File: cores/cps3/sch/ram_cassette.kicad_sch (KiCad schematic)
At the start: 13 parts

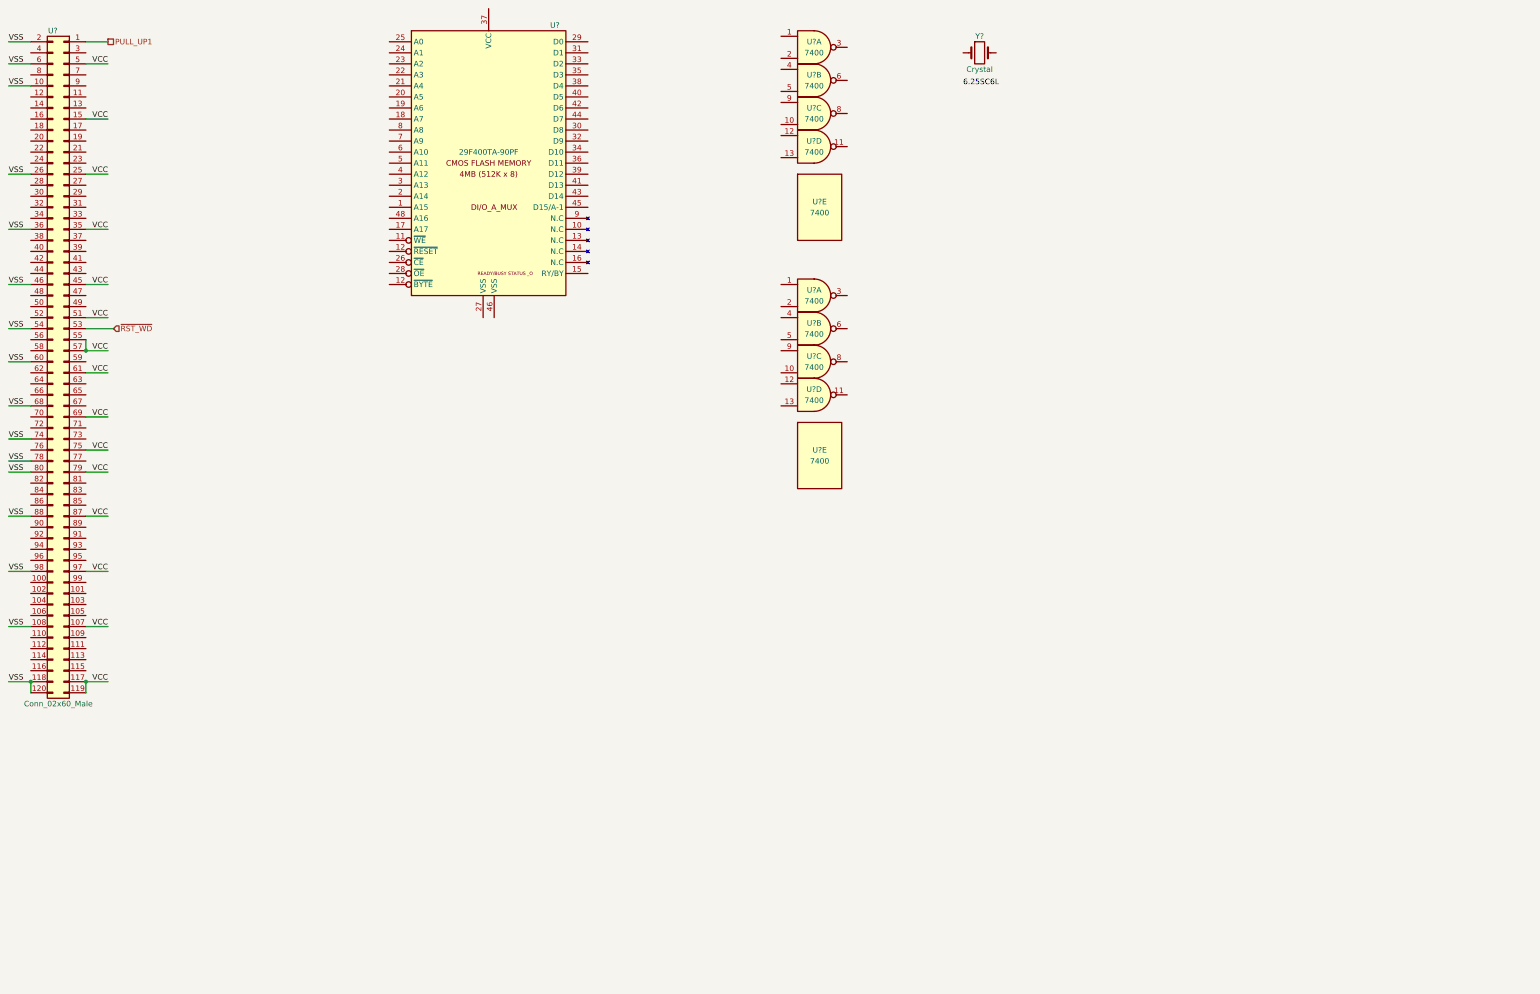
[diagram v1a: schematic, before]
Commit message: wip_cassette
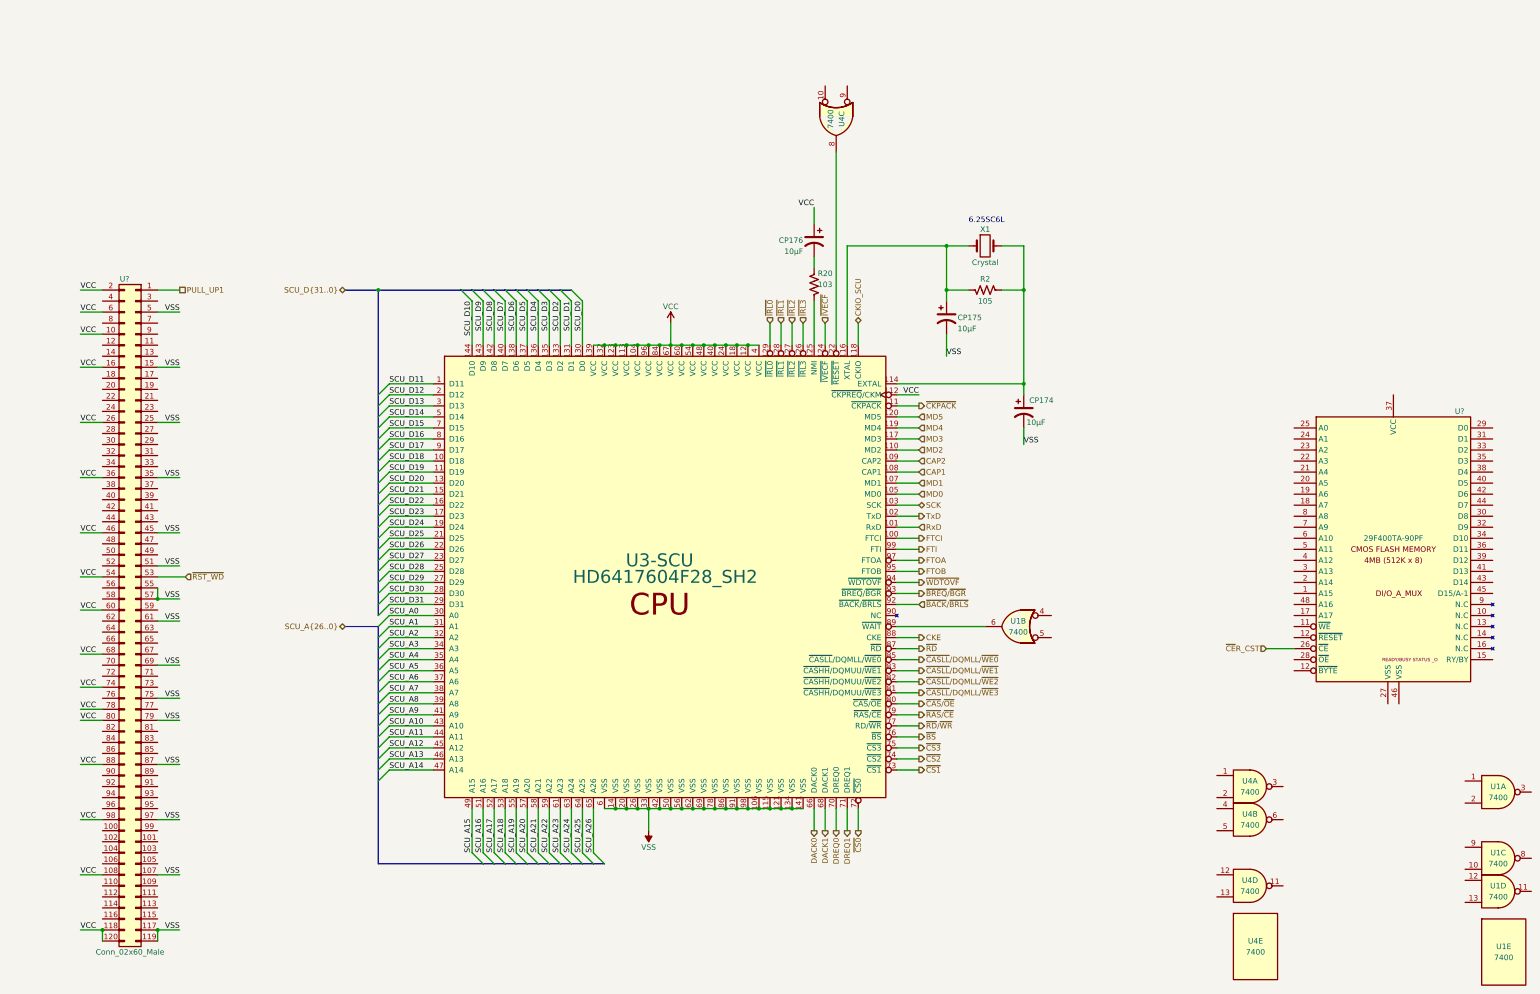
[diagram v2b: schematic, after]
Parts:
- added CP174, CP175, CP176: 10μF, symbol Device:C_Polarized_US
- added R2: 105, symbol Device:R_US
- added R20: 103, symbol Device:R_US
- added U3-SCU: HD6417604F28_SH2, symbol arcade:HD6417604F28_SH2
- gave numbers to parts that had none: 3
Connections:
- net VCC: now also U?.10 (Pin_10), U?.108 (Pin_108), U?.118 (Pin_118), U?.120 (Pin_120), U?.16 (Pin_16), U?.2, U?.26 (Pin_26), U?.36 (Pin_36), U?.46 (Pin_46), U?.54 (Pin_54), U?.6, U?.60 (Pin_60), U?.68 (Pin_68), U?.74 (Pin_74), U?.78 (Pin_78), U?.80 (Pin_80), U?.88 (Pin_88), U?.98 (Pin_98), CP176.1, U3-SCU.104 (VCC), U3-SCU.112 (~{CKPREQ}/CKM), U3-SCU.113 (VCC), U3-SCU.12 (VCC), U3-SCU.123 (VCC), U3-SCU.132 (VCC), U3-SCU.139 (VCC), U3-SCU.18 (VCC), U3-SCU.24 (VCC), U3-SCU.4 (VCC), U3-SCU.40 (VCC), U3-SCU.48 (VCC), U3-SCU.54 (VCC), U3-SCU.60 (VCC), U3-SCU.67 (VCC), U3-SCU.84 (VCC), U3-SCU.96 (VCC); no longer U?.107 (Pin_107), U?.117 (Pin_117), U?.119 (Pin_119), U?.15 (Pin_15), U?.25 (Pin_25), U?.35 (Pin_35), U?.45 (Pin_45), U?.5 (Pin_5), U?.51 (Pin_51), U?.55 (Pin_55), U?.57 (Pin_57), U?.61 (Pin_61), U?.69 (Pin_69), U?.75 (Pin_75), U?.79 (Pin_79), U?.87 (Pin_87), U?.97 (Pin_97)
- net VSS: now also U?.107 (Pin_107), U?.117 (Pin_117), U?.119 (Pin_119), U?.15 (Pin_15), U?.25 (Pin_25), U?.35 (Pin_35), U?.45 (Pin_45), U?.5 (Pin_5), U?.51 (Pin_51), U?.55 (Pin_55), U?.57 (Pin_57), U?.61 (Pin_61), U?.69 (Pin_69), U?.75 (Pin_75), U?.79 (Pin_79), U?.87 (Pin_87), U?.97 (Pin_97), CP174.2, CP175.2, U3-SCU.106 (VSS), U3-SCU.115 (VSS), U3-SCU.121 (VSS), U3-SCU.134 (VSS), U3-SCU.14 (VSS), U3-SCU.141 (VSS), U3-SCU.20 (VSS), U3-SCU.26 (VSS), U3-SCU.33 (VSS), U3-SCU.42 (VSS), U3-SCU.50 (VSS), U3-SCU.56 (VSS), U3-SCU.6 (VSS), U3-SCU.62 (VSS), U3-SCU.69 (VSS), U3-SCU.78 (VSS), U3-SCU.86 (VSS), U3-SCU.91 (VSS), U3-SCU.98 (VSS); no longer U?.10 (Pin_10), U?.108 (Pin_108), U?.118 (Pin_118), U?.120 (Pin_120), U?.2, U?.26 (Pin_26), U?.36 (Pin_36), U?.46 (Pin_46), U?.54 (Pin_54), U?.6, U?.60 (Pin_60), U?.68 (Pin_68), U?.74 (Pin_74), U?.78 (Pin_78), U?.80 (Pin_80), U?.88 (Pin_88), U?.98 (Pin_98)
- net at U1.6: now also U3-SCU.89 (~{WAIT})
- net at X1.1: now also CP175.1, R2.1, U3-SCU.116 (XTAL)
- net at X1.2: now also CP174.1, R2.2, U3-SCU.114 (EXTAL)
- net at U4.8: now also U3-SCU.122 (~{RESET})
- net ~{CE}R_CST: now reaches U?.26 (~{CE})
- new net: CP176.2, R20.2
- new net: R20.1, U3-SCU.125 (NMI)
- new net CAP1: U3-SCU.108 (CAP1)
- new net CAP2: U3-SCU.109 (CAP2)
- new net CKE: U3-SCU.88 (CKE)
- new net CKIO_SCU: U3-SCU.118 (CKIO)
- new net DACK0: U3-SCU.66 (DACK0)
- new net DACK1: U3-SCU.68 (DACK1)
- new net DREQ0: U3-SCU.70 (DREQ0)
- new net DREQ1: U3-SCU.71 (DREQ1)
- new net FTCI: U3-SCU.100 (FTCI)
- new net FTI: U3-SCU.99 (FTI)
- new net FTOA: U3-SCU.97 (FTOA)
- new net FTOB: U3-SCU.95 (FTOB)
- new net MD0: U3-SCU.105 (MD0)
- new net MD1: U3-SCU.107 (MD1)
- new net MD2: U3-SCU.110 (MD2)
- new net MD3: U3-SCU.117 (MD3)
- new net MD4: U3-SCU.119 (MD4)
- new net MD5: U3-SCU.120 (MD5)
- new net RxD: U3-SCU.101 (RxD)
- new net SCK: U3-SCU.103 (SCK)
- new net SCU_A0: U3-SCU.30 (A0)
- new net SCU_A1: U3-SCU.31 (A1)
- new net SCU_A10: U3-SCU.43 (A10)
- new net SCU_A11: U3-SCU.44 (A11)
- new net SCU_A12: U3-SCU.45 (A12)
- new net SCU_A13: U3-SCU.46 (A13)
- new net SCU_A14: U3-SCU.47 (A14)
- new net SCU_A15: U3-SCU.49 (A15)
- new net SCU_A16: U3-SCU.51 (A16)
- new net SCU_A17: U3-SCU.52 (A17)
- new net SCU_A18: U3-SCU.53 (A18)
- new net SCU_A19: U3-SCU.55 (A19)
- new net SCU_A2: U3-SCU.32 (A2)
- new net SCU_A20: U3-SCU.57 (A20)
- new net SCU_A21: U3-SCU.58 (A21)
- new net SCU_A22: U3-SCU.59 (A22)
- new net SCU_A23: U3-SCU.61 (A23)
- new net SCU_A24: U3-SCU.63 (A24)
- new net SCU_A25: U3-SCU.64 (A25)
- new net SCU_A26: U3-SCU.65 (A26)
- new net SCU_A3: U3-SCU.34 (A3)
- new net SCU_A4: U3-SCU.35 (A4)
- new net SCU_A5: U3-SCU.36 (A5)
- new net SCU_A6: U3-SCU.37 (A6)
- new net SCU_A7: U3-SCU.38 (A7)
- new net SCU_A8: U3-SCU.39 (A8)
- new net SCU_A9: U3-SCU.41 (A9)
- new net SCU_D0: U3-SCU.130 (D0)
- new net SCU_D1: U3-SCU.131 (D1)
- new net SCU_D10: U3-SCU.144 (D10)
- new net SCU_D11: U3-SCU.1 (D11)
- new net SCU_D12: U3-SCU.2 (D12)
- new net SCU_D13: U3-SCU.3 (D13)
- new net SCU_D14: U3-SCU.5 (D14)
- new net SCU_D15: U3-SCU.7 (D15)
- new net SCU_D16: U3-SCU.8 (D16)
- new net SCU_D17: U3-SCU.9 (D17)
- new net SCU_D18: U3-SCU.10 (D18)
- new net SCU_D19: U3-SCU.11 (D19)
- new net SCU_D2: U3-SCU.133 (D2)
- new net SCU_D20: U3-SCU.13 (D20)
- new net SCU_D21: U3-SCU.15 (D21)
- new net SCU_D22: U3-SCU.16 (D22)
- new net SCU_D23: U3-SCU.17 (D23)
- new net SCU_D24: U3-SCU.19 (D24)
- new net SCU_D25: U3-SCU.21 (D25)
- new net SCU_D26: U3-SCU.22 (D26)
- new net SCU_D27: U3-SCU.23 (D27)
- new net SCU_D28: U3-SCU.25 (D28)
- new net SCU_D29: U3-SCU.27 (D29)
- new net SCU_D3: U3-SCU.135 (D3)
- new net SCU_D30: U3-SCU.28 (D30)
- new net SCU_D31: U3-SCU.29 (D31)
- new net SCU_D4: U3-SCU.136 (D4)
- new net SCU_D5: U3-SCU.137 (D5)
- new net SCU_D6: U3-SCU.138 (D6)
- new net SCU_D7: U3-SCU.140 (D7)
- new net SCU_D8: U3-SCU.142 (D8)
- new net SCU_D9: U3-SCU.143 (D9)
- new net TxD: U3-SCU.102 (TxD)
- new net ~{BACK}/~{BRLS}: U3-SCU.92 (~{BACK}/~{BRLS})
- new net ~{BREQ}/~{BGR}: U3-SCU.93 (~{BREQ}/~{BGR})
- new net ~{BS}: U3-SCU.76 (~{BS})
- new net ~{CASLL}/DQMLL/~{WE0}: U3-SCU.85 (~{CASLL}/DQMLL/~{WE0})
- new net ~{CASLL}/DQMLL/~{WE1}: U3-SCU.83 (~{CASHH}/DQMUU/~{WE1})
- new net ~{CASLL}/DQMLL/~{WE2}: U3-SCU.82 (~{CASHH}/DQMUU/~{WE2})
- new net ~{CASLL}/DQMLL/~{WE3}: U3-SCU.81 (~{CASHH}/DQMUU/~{WE3})
- new net ~{CAS}/~{OE}: U3-SCU.80 (~{CAS}/~{OE})
- new net ~{CKPACK}: U3-SCU.111 (~{CKPACK})
- new net ~{CS0}: U3-SCU.72 (~{CS0})
- new net ~{CS1}: U3-SCU.73 (~{CS1})
- new net ~{CS2}: U3-SCU.74 (~{CS2})
- new net ~{CS3}: U3-SCU.75 (~{CS3})
- new net ~{IRL0}: U3-SCU.129 (~{IRL0})
- new net ~{IRL1}: U3-SCU.128 (~{IRL1})
- new net ~{IRL2}: U3-SCU.127 (~{IRL2})
- new net ~{IRL3}: U3-SCU.126 (~{IRL3})
- new net ~{IVECF}: U3-SCU.124 (~{IVECF})
- new net ~{RAS}/~{CE}: U3-SCU.79 (~{RAS}/~{CE})
- new net ~{RD}: U3-SCU.87 (~{RD})
- new net ~{RD}/~{WR}: U3-SCU.77 (RD/~{WR})
- new net ~{WDTOVF}: U3-SCU.94 (~{WDTOVF})
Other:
- moved on the sheet: U1A, U1C, U1D, U1E, U4A, U4B, U4D, U4E, U?, X1
